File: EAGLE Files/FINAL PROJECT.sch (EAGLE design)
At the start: 15 parts, among them J1 BATTERY, U1 9_to_3.3_VREG

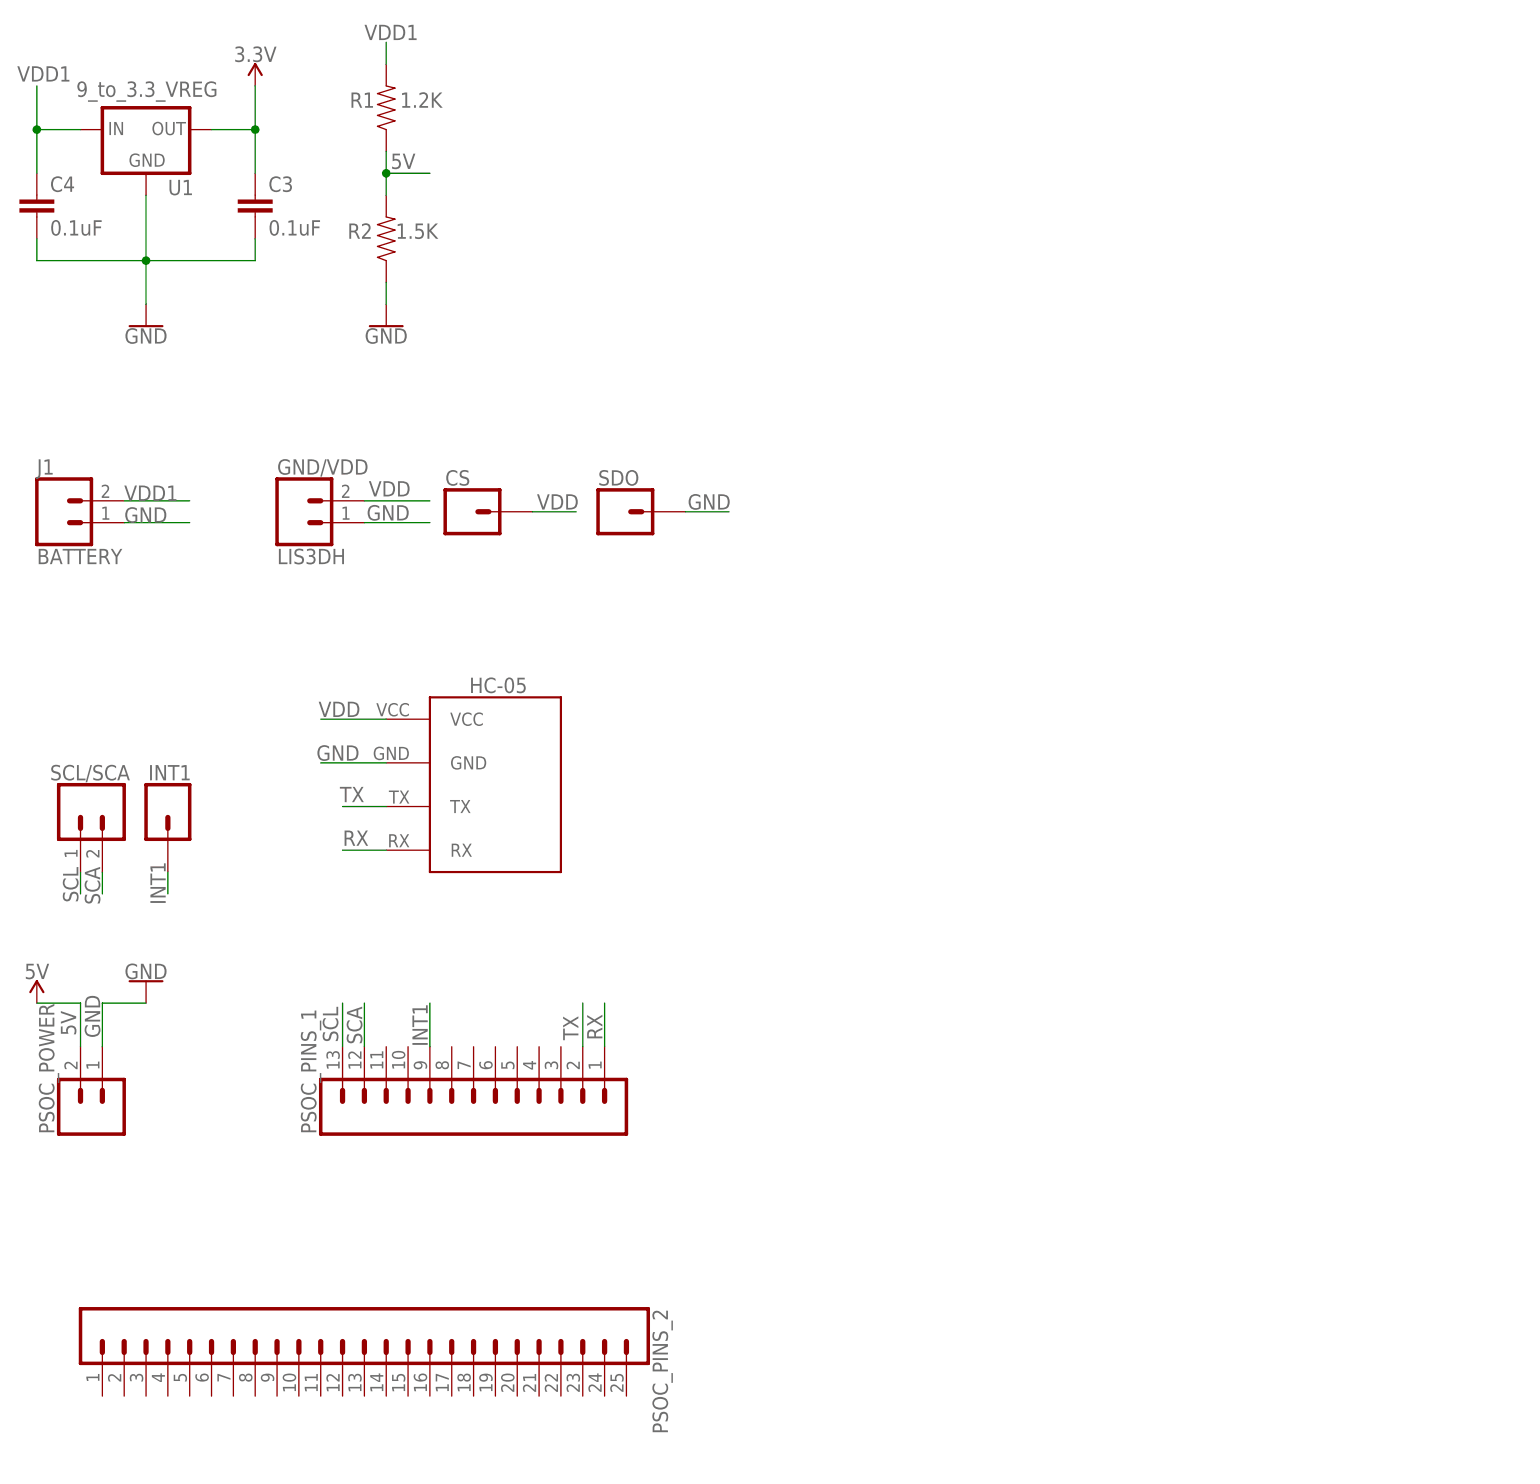
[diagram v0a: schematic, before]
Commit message: FS and So code
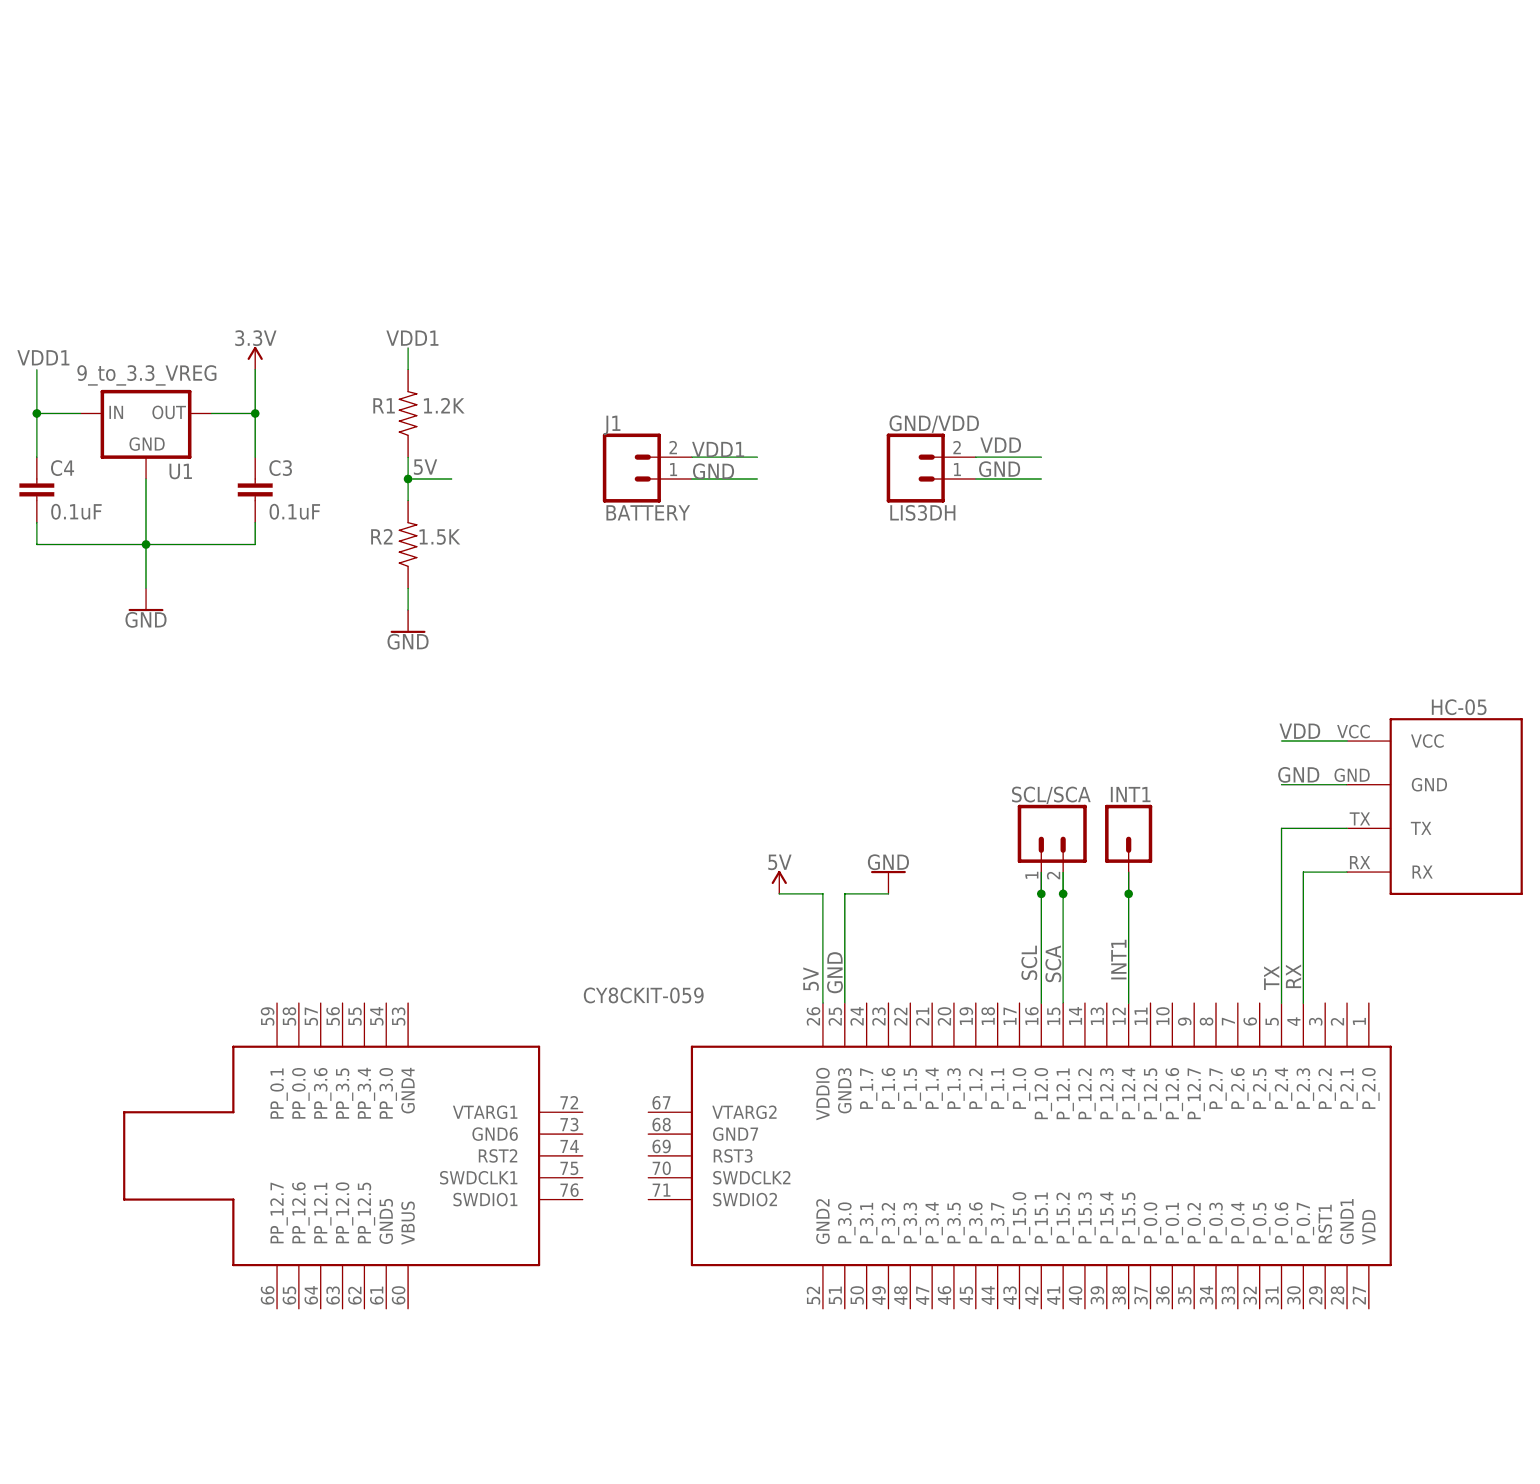
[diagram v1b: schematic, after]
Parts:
- removed CS, SDO: (no value), SparkFun-Connectors:CONN_01
- removed PSOC_PINS_1: (no value), SparkFun-Connectors:CONN_13
- removed PSOC_PINS_2: (no value), SparkFun-Connectors:CONN_25
- removed PSOC_POWER: (no value), SparkFun-Connectors:CONN_02
- added U$1: CY8CKIT-059, CYKIT:CY8CKIT-059
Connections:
- net 5V: now also U$1.VDDIO; no longer PSOC_POWER.2
- net GND: now also U$1.GND3; no longer PSOC_POWER.1, SDO.1
- net INT1: now also U$1.P_12.4; no longer PSOC_PINS_1.9
- net RX: now also U$1.P_2.3; no longer PSOC_PINS_1.1
- net SCA: now also U$1.P_12.1; no longer PSOC_PINS_1.12
- net SCL: now also U$1.P_12.0; no longer PSOC_PINS_1.13
- net TX: now also U$1.P_2.4; no longer PSOC_PINS_1.2
- net VDD: no longer CS.1
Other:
- moved on the sheet: C3, C4, GND/VDD, HC-05, INT1, J1, R1, R2, SCL/SCA, U1

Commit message: update - EAGLE files
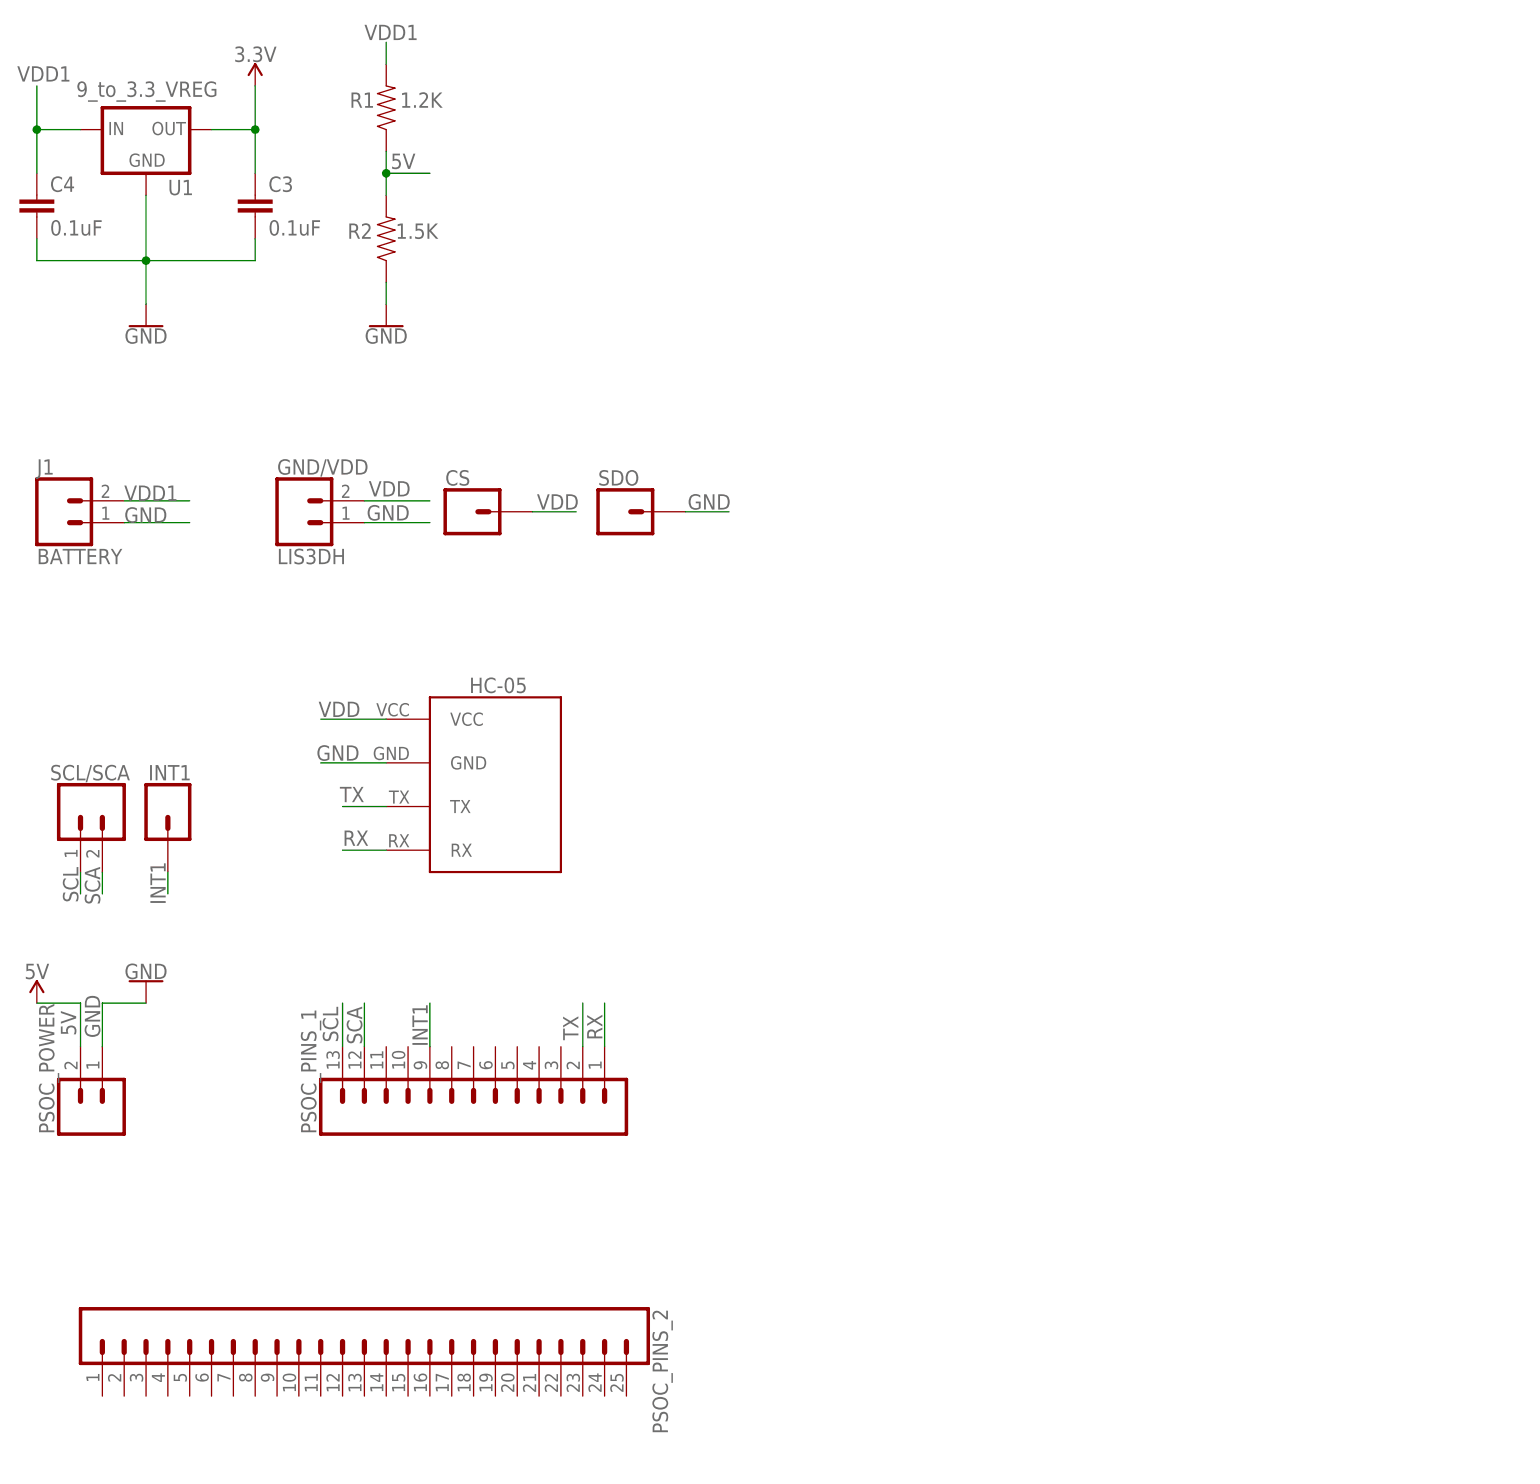
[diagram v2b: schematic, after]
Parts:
- removed U$1: CY8CKIT-059, CYKIT:CY8CKIT-059
- added CS, SDO: (no value), SparkFun-Connectors:CONN_01
- added PSOC_PINS_1: (no value), SparkFun-Connectors:CONN_13
- added PSOC_PINS_2: (no value), SparkFun-Connectors:CONN_25
- added PSOC_POWER: (no value), SparkFun-Connectors:CONN_02
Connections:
- net 5V: now also PSOC_POWER.2; no longer U$1.VDDIO
- net GND: now also PSOC_POWER.1, SDO.1; no longer U$1.GND3
- net INT1: now also PSOC_PINS_1.9; no longer U$1.P_12.4
- net RX: now also PSOC_PINS_1.1; no longer U$1.P_2.3
- net SCA: now also PSOC_PINS_1.12; no longer U$1.P_12.1
- net SCL: now also PSOC_PINS_1.13; no longer U$1.P_12.0
- net TX: now also PSOC_PINS_1.2; no longer U$1.P_2.4
- net VDD: now also CS.1
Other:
- moved on the sheet: C3, C4, GND/VDD, HC-05, INT1, J1, R1, R2, SCL/SCA, U1
